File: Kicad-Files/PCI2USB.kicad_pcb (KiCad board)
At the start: 4 copper layers, 22 x 80 mm, 107 parts, among them J2 USB_9PIN_Internal, U1 TPS61023, U2 TUSB7320, U3 TPS74401, U4 TPS2560, Y1 48 MHz

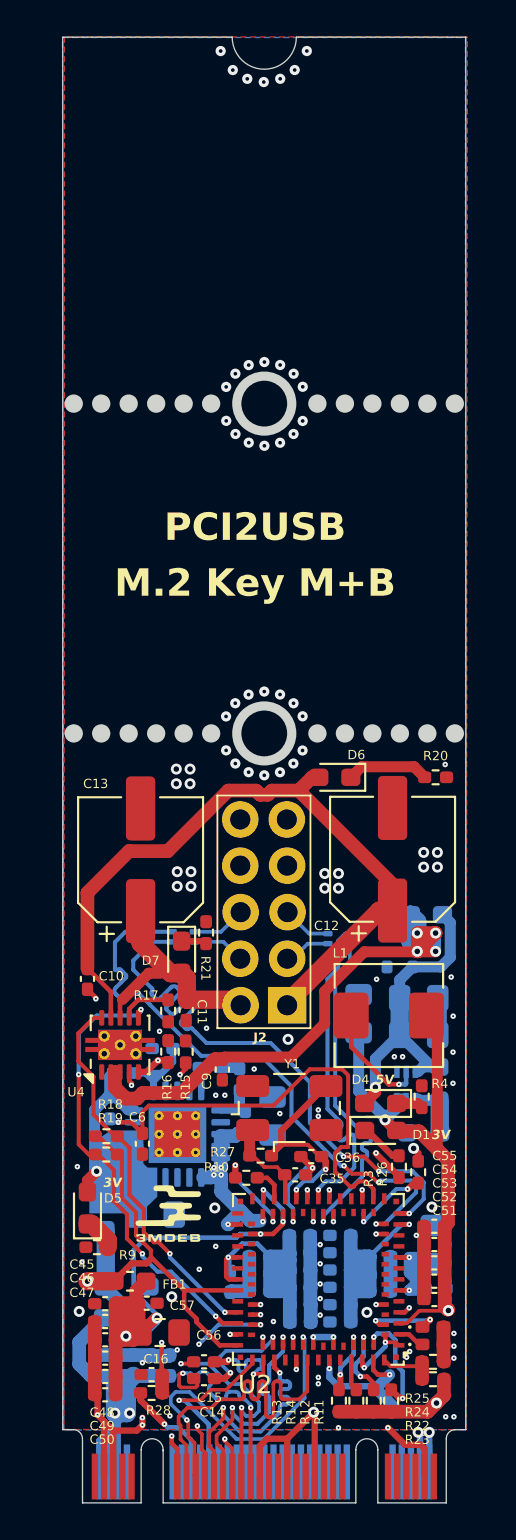
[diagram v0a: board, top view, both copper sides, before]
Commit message: Redesigned PCB compliant with PCI and SS USB standards
Signed-off-by: Jakub Sobota <jakub.sobota@3mdeb.com>
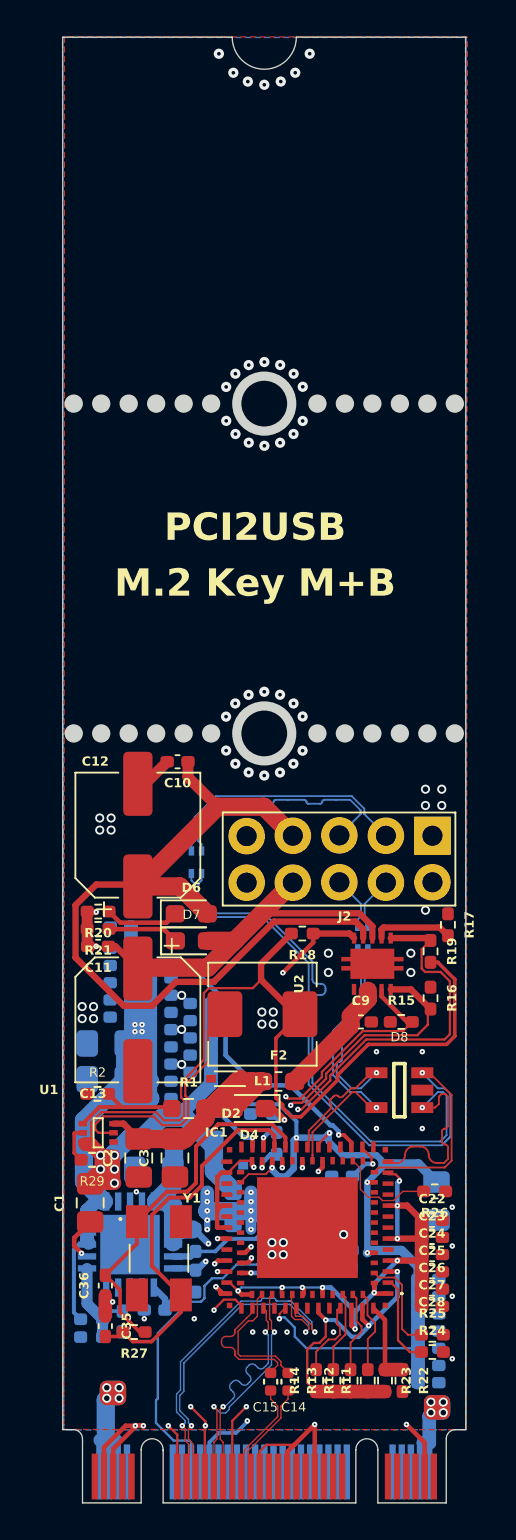
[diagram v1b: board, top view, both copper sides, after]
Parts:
- removed D1, D5: LED, LED_SMD:LED_0603_1608Metric_Pad1.05x0.95mm_HandSolder
- removed G***: LOGO, LOGO
- removed R3: 680 Ohm, Resistor_SMD:R_0402_1005Metric_Pad0.72x0.64mm_HandSolder
- removed R9: 330 Ohm, Resistor_SMD:R_0402_1005Metric_Pad0.72x0.64mm_HandSolder
- removed U4: TPS2560, Package_SON:VSON-10-1EP_3x3mm_P0.5mm_EP1.65x2.4mm_ThermalVias
- added D8: ESDS304DBVR, ESDS304:ESDS304DBVR, F.Cu at (153.5, 108.1)
- added IC1: TUSB7320, TUSB7320:TUSB7320RKMT, F.Cu at (148.5, 115.6)
- added R29: 100 KOhm, Resistor_SMD:R_0402_1005Metric_Pad0.72x0.64mm_HandSolder, F.Cu at (136.8, 111.9)
- C1: value 10 μF -> 22 μF; moved to F.Cu
- C14, C15: footprint Capacitor_SMD:C_0402_1005Metric_Pad0.74x0.62mm_HandSolder -> Capacitor_SMD:C_0402_1005Metric
- C16, C45, C46, C47, C48, C49, C50, C51, C52, C53, C54, C55, C56, C57, C6, FB1, R10, R28, R4: moved to B.Cu
- C2, C22, C23, C24, C25, C26, C27, C3, F2, R1: moved to F.Cu
- D2: value 6V/5A -> 6V/9V/5A; footprint Diode_SMD:D_SOD-523 -> PJSD0XTS-AU:PJSD0XTS-AU; moved to F.Cu
- D3: value 4V/5A -> 4V/6.5V/5A; footprint Diode_SMD:D_SOD-323_HandSoldering -> PJSD0XTS-AU:PJSD0XTS-AU
- FL1, FL2: value 90 Ohm -> 90 Ohm 160mA; footprint Filters:MCZ1210AH_CP -> MCZ1210AH900L2TA0G:MCZ1210AH201L2TA0G
- J1: value ~ -> M.2 Edge Connector; footprint M2_Edge_connector:M.2_KEY_M_B -> Connectors:M.2_KEY_M_B
- R2: footprint Resistor_SMD:R_0603_1608Metric_Pad0.98x0.95mm_HandSolder -> Resistor_SMD:R_0402_1005Metric_Pad0.72x0.64mm_HandSolder; moved to F.Cu
- R24, R25: footprint LED_SMD:LED_0402_1005Metric_Pad0.77x0.64mm_HandSolder -> Resistor_SMD:R_0402_1005Metric_Pad0.72x0.64mm_HandSolder
- U1: value TPS61023 -> TPS61023DRLR; footprint DC-DC:TPS61023 -> TPS61023:TPS61023DRLR; moved to F.Cu
- U2: value TUSB7320 -> TPS2560DRC; footprint TUSB7320:Texas_tusb7320 -> TPS2560:TPS2560DRCT
- U3: footprint Package_DFN_QFN:Texas_RGW0020A_VQFN-20-1EP_5x5mm_P0.65mm_EP3.15x3.15mm_ThermalVias -> TPS74401:TPS74401RGWRM3
- Y1: footprint Crystal:Crystal_SMD_Abracon_ABM3B-4Pin_5.0x3.2mm -> ABM3B:ABM3B-48.000MHZ-B2-T
- moved C28 22.0 mm to (138.3, 99.2), turned to 180 degrees
- moved C44 21.2 mm to (140.5, 102.0), turned to 0 degrees
- moved R19 20.9 mm to (155.2, 100.5), turned to -90 degrees
- moved C32 20.5 mm to (138.3, 103.2)
- moved C29 20.1 mm to (138.3, 100.3), turned to 180 degrees
- moved C43 20.1 mm to (140.5, 102.9)
- moved C34 20.0 mm to (137.5, 107.5), turned to 180 degrees
- moved C40 20.0 mm to (140.5, 105.7)
- moved R20 19.8 mm to (137.1, 98.3), turned to 180 degrees
- moved C53 19.1 mm to (142.7, 103.3)
- moved C33 19.0 mm to (138.3, 104.1)
- moved C42 18.6 mm to (140.5, 103.8)
- moved C30 18.5 mm to (138.3, 101.3), turned to 180 degrees
- moved C49 18.4 mm to (155.1, 118.4), turned to 0 degrees
- moved C48 18.0 mm to (155.1, 119.3), turned to 0 degrees
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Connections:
- C1 pad 1: +3.3V -> GND
- C1 pad 2: GND -> +3.3V
- C35 pad 1: Net-(U2-VSS_OSC) -> Net-(IC1-VSS_OSC)
- C35 pad 2: Net-(U2-XI) -> Net-(IC1-XI)
- C36 pad 1: Net-(U2-VSS_OSC) -> Net-(IC1-VSS_OSC)
- C36 pad 2: Net-(U2-XO) -> Net-(IC1-XO)
- D3 pad 1: GND -> +3.3V
- D3 pad 2: +3.3V -> GND
- FL1 pad 1: Net-(FL1-Pad1) -> DP1
- FL1 pad 2: Net-(FL1-Pad2) -> DM1
- FL1 pad 3: DP2 -> Net-(FL1-Pad3)
- FL1 pad 4: DM2 -> Net-(FL1-Pad4)
- FL2 pad 1: DM1 -> DM2
- FL2 pad 2: DP1 -> DP2
- J1 pad 47: PCIE_RXP -> PCIE_RXN
- J1 pad 49: PCIE_RXN -> PCIE_RXP
- J2 pad 1: DS1_VBUS -> GND
- J2 pad 2: DS2_VBUS -> GND
- J2 pad 4: Net-(FL1-Pad1) -> Net-(FL1-Pad3)
- J2 pad 6: Net-(FL1-Pad2) -> Net-(FL1-Pad4)
- J2 pad 7: GND -> DS1_VBUS
- J2 pad 8: GND -> DS2_VBUS
- R10 pad 1: Net-(U2-R1EXT) -> Net-(IC1-R1EXT)
- R10 pad 2: Net-(U2-R1EXTRTN) -> Net-(IC1-R1EXTRTN)
- R11 pad 2: Net-(U2-GPIO3) -> Net-(IC1-GPIO3)
- R12 pad 2: Net-(U2-GPIO2) -> Net-(IC1-GPIO2)
- R13 pad 2: Net-(U2-GPIO1) -> Net-(IC1-GPIO1)
- R14 pad 2: Net-(U2-GPIO0) -> Net-(IC1-GPIO0)
- R17 pad 2: Net-(U4-ILM) -> Net-(U2-ILIM)
- R22 pad 1: Net-(U2-AUX_DET) -> Net-(IC1-AUX_DET)
- R23 pad 1: Net-(U2-AUX_DET) -> Net-(IC1-AUX_DET)
- R24 pad 1: Net-(U2-SDA) -> Net-(IC1-SDA)
- R25 pad 1: Net-(U2-SCL) -> Net-(IC1-SCL)
- R26 pad 2: Net-(U2-FREQSEL) -> Net-(IC1-FREQSEL)
- R27 pad 1: Net-(U2-XO) -> Net-(IC1-XO)
- R27 pad 2: Net-(U2-XI) -> Net-(IC1-XI)
- U1 pad 2: +3.3V -> Net-(U1-EN)
- Y1 pad 1: Net-(U2-XI) -> Net-(IC1-XO)
- Y1 pad 3: Net-(U2-XO) -> Net-(IC1-XI)
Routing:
- net +5V: track 39.0 -> 6.30 mm, vias 4 -> 0
- net Net-(IC1-XI): track 0.00 -> 21.2 mm
- net Net-(C17-Pad1): track 47.3 -> 68.2 mm, vias 4 -> 18
- net Net-(IC1-XO): track 0.00 -> 20.1 mm
- net GND: track 63.3 -> 43.5 mm, vias 108 -> 89
- net +3.3V: track 108.0 -> 127.4 mm, vias 6 -> 10
- net Net-(IC1-VSS_OSC): track 0.00 -> 17.6 mm, vias 0 -> 2
- net Net-(J1-PEWAKE#): track 5.80 -> 22.0 mm, vias 1 -> 0
- net PERSTZ: track 9.80 -> 21.3 mm, vias 1 -> 2
- net Net-(U2-XO): track 11.5 -> 0.00 mm, vias 2 -> 0
- net Net-(FL2-Pad3): track 2.69 -> 13.9 mm
- net GRSTZ: track 26.3 -> 15.3 mm
- net Net-(FL2-Pad4): track 3.06 -> 13.9 mm
- net +1.1V: track 120.4 -> 131.1 mm, vias 21 -> 18
- net OVERCUR2Z: track 25.2 -> 32.9 mm, vias 4 -> 2
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
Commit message: Fixed reversed 9 pin connector
Signed-off-by: Jakub Sobota <jakub.sobota@3mdeb.com>
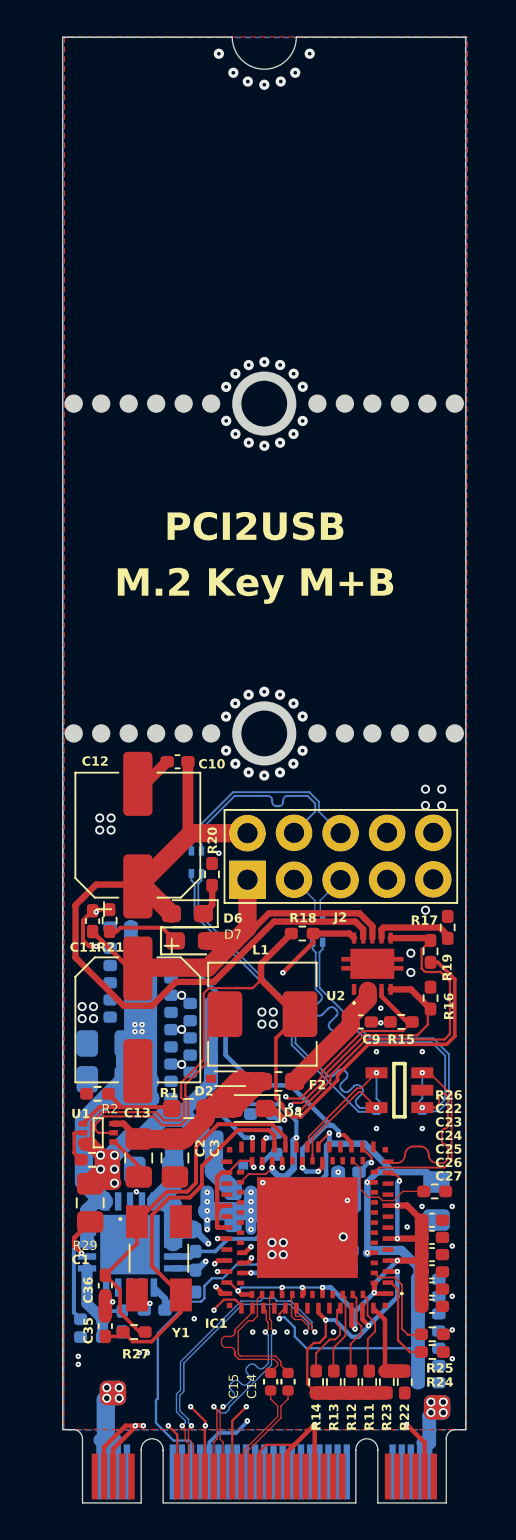
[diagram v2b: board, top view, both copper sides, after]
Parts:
- moved FL1 9.97 mm to (142.4, 95.6)
- moved FL2 7.60 mm to (149.1, 99.4)
- moved R20 6.54 mm to (143.3, 96.3), turned to 90 degrees
- moved C11 1.41 mm to (136.8, 98.8), turned to 90 degrees
- moved R21 0.78 mm to (137.7, 98.8), turned to 90 degrees
- moved C6 0.42 mm to (150.8, 112.5)
- moved D6 0.21 mm to (142.0, 98.4), turned to 180 degrees
- moved R22 0.15 mm to (153.8, 124.0)
- moved R17 0.14 mm to (156.2, 99.2)
- moved R23 0.13 mm to (152.8, 124.0)
- moved R11 0.11 mm to (151.9, 124.0)
- moved R12 0.09 mm to (150.9, 124.0)
- moved R13 0.08 mm to (149.9, 124.0)
- moved R14 0.08 mm to (149.0, 124.0)
- moved C21 0.05 mm to (150.0, 114.3)
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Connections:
- net DM2 renamed D2-
- net DP2 renamed D2+
- J2 pad 1: GND -> DS2_VBUS
- J2 pad 2: GND -> DS1_VBUS
- J2 pad 7: DS1_VBUS -> GND
- J2 pad 8: DS2_VBUS -> GND
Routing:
- net D2+: track 40.2 -> 28.2 mm
- net D2-: track 39.4 -> 28.1 mm
- net Net-(FL2-Pad4): track 13.9 -> 2.71 mm
- net Net-(FL2-Pad3): track 13.9 -> 2.68 mm
- net DP1: track 17.0 -> 26.2 mm
- net DM1: track 17.0 -> 26.1 mm
- net Net-(FL1-Pad4): track 2.97 -> 11.4 mm
- net Net-(FL1-Pad3): track 2.94 -> 11.3 mm
- net DS1_VBUS: track 44.5 -> 39.7 mm
- net GND: track 43.5 -> 47.9 mm, vias 89 -> 100
- net +1.1V: track 131.1 -> 134.2 mm
- net VDDA_3P3: track 50.4 -> 52.9 mm
- net Net-(D6-K): track 4.06 -> 1.64 mm
- net DS2_VBUS: track 21.3 -> 22.7 mm
